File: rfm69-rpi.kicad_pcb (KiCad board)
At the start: 2 copper layers, 65 x 56 mm, 21 parts, among them IC1 RFM69, IC2 RFM69, IC3 RFM69, IC4 RFM69, IC5 NCP1117, IC6 74HC139, J1 RPi_GPIO, P1 COAX, P2 COAX, P3 COAX, P4 COAX, P5 POWER, U1 1-Wire, U2 1-Wire

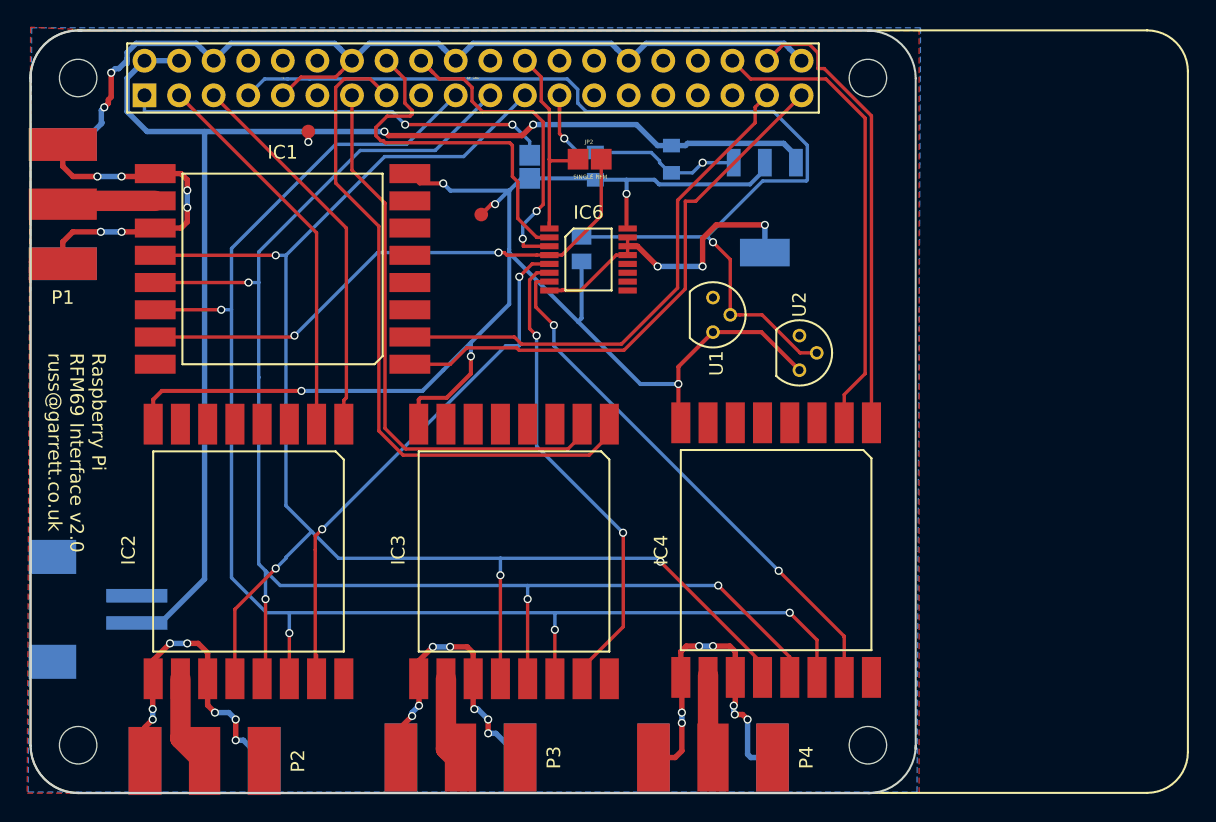
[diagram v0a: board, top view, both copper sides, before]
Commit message: Version 2.0
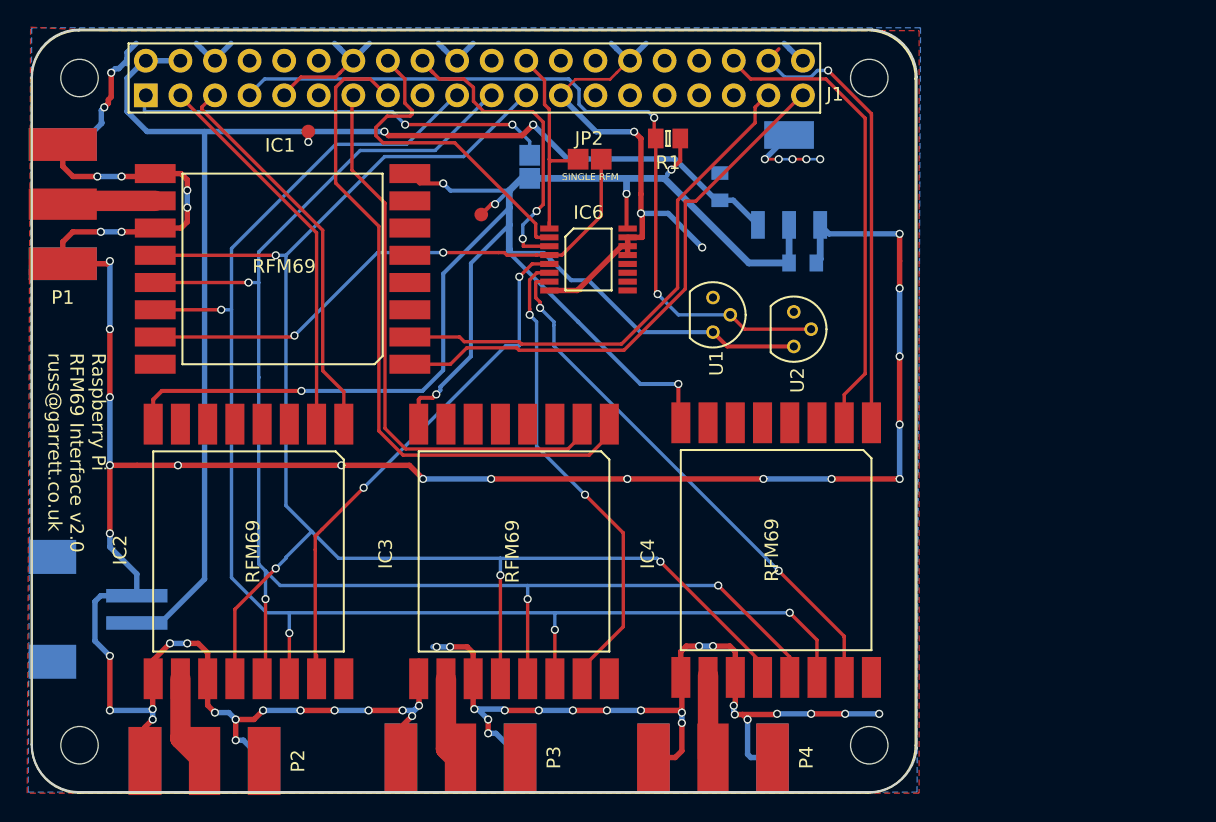
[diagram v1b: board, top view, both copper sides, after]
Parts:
- J1: footprint tinkerforge:raspberrypi2 -> russ:raspberrypi2
- R1: moved to F.Cu
- moved C2 16.8 mm to (152.2, 82.6), turned to 0 degrees
- moved R1 10.3 mm to (142.3, 73.4), turned to 180 degrees
- moved C1 4.09 mm to (146.1, 77.0), turned to 90 degrees
- moved IC5 2.70 mm to (151.2, 76.5), turned to 180 degrees
- moved U2 1.79 mm to (151.6, 86.2)
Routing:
- net Earth: track 211.6 -> 344.8 mm, vias 34 -> 70
- net +3V3: track 121.1 -> 150.4 mm, vias 6 -> 7
- net ONEWIRE: track 79.0 -> 57.5 mm, vias 1 -> 2
- net Net-(IC6-Pad2): track 27.1 -> 24.7 mm
- net +5V: track 99.3 -> 98.1 mm
- net RESET2: track 28.3 -> 28.8 mm
- net RESET4: track 33.6 -> 33.5 mm, vias 0 -> 1
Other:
- outline, holes or cut-outs redrawn
